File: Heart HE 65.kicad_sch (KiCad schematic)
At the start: 61 parts, among them J6 Conn_01x04, SW1 SW_Push, U1 PRTR5V0U2X, U19 AP2112K-3.3, U27 AT32F405KxU7-4, U63 AMS1117-3.3, U85 TPS63001, Y1 12Mhz (15p)

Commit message: Fix Component order part overwrite
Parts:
- C165, C20, C21, C25, C26, C32, C6, C8: LCSC C52923 -> (none)
- USB1: LCSC Part Number C165948 -> (none)
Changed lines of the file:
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@@
 			)
 		)
-		(property "LCSC" "C52923"
-			(at 140.97 139.7 0)
-			(effects
-				(font
-					(size 1.27 1.27)
-				)
-				(hide yes)
-			)
-		)
 		(pin "1"
 		)
@@
 			)
 		)
-		(property "LCSC" "C52923"
-			(at 151.13 139.7 0)
-			(effects
-				(font
-					(size 1.27 1.27)
-				)
-				(hide yes)
-			)
-		)
 		(pin "1"
 		)
@@
 			)
 		)
-		(property "LCSC" "C52923"
-			(at 217.17 105.41 0)
-			(effects
-				(font
-					(size 1.27 1.27)
-				)
-				(hide yes)
-			)
-		)
 		(pin "1"
 		)
@@
 			)
 		)
-		(property "LCSC" "C52923"
-			(at 260.985 99.695 0)
-			(effects
-				(font
-					(size 1.27 1.27)
-				)
-				(hide yes)
-			)
-		)
 		(pin "1"
 		)
@@
 			)
 		)
-		(property "LCSC" "C52923"
-			(at 153.67 153.67 0)
-			(effects
-				(font
-					(size 1.27 1.27)
-				)
-				(hide yes)
-			)
-		)
 		(pin "1"
 		)
@@
 			)
 		)
-		(property "LCSC" "C52923"
-			(at 158.75 153.67 0)
-			(effects
-				(font
-					(size 1.27 1.27)
-				)
-				(hide yes)
-			)
-		)
 		(pin "1"
 		)
@@
 			)
 		)
-		(property "LCSC" "C52923"
-			(at 137.16 186.69 0)
-			(effects
-				(font
-					(size 1.27 1.27)
-				)
-				(hide yes)
-			)
-		)
 		(pin "1"
 		)
@@
 			)
 		)
-		(property "LCSC" "C52923"
-			(at 162.56 186.69 0)
-			(effects
-				(font
-					(size 1.27 1.27)
-				)
-				(hide yes)
-			)
-		)
 		(pin "1"
 		)
@@
 			)
 		)
-		(property "LCSC" "C52923"
-			(at 257.175 99.695 0)
-			(effects
-				(font
-					(size 1.27 1.27)
-				)
-				(hide yes)
-			)
-		)
 		(pin "1"
 		)
@@
 			)
 		)
-		(property "LCSC" "C52923"
-			(at 200.025 150.495 0)
-			(effects
-				(font
-					(size 1.27 1.27)
-				)
-				(hide yes)
-			)
-		)
 		(pin "1"
 		)
@@
 			)
 		)
-		(property "LCSC" "C52923"
-			(at 181.61 150.495 0)
-			(effects
-				(font
-					(size 1.27 1.27)
-				)
-				(hide yes)
-			)
-		)
 		(pin "1"
 		)
@@
 			)
 		)
-		(property "LCSC Part Number" "C165948"
-			(at 22.86 199.39 0)
-			(effects
-				(font
-					(size 1.27 1.27)
-				)
-				(hide yes)
-			)
-		)
 		(pin "1"
 		)
@@
 			)
 		)
-		(property "LCSC" "C52923"
-			(at 210.82 96.52 0)
-			(effects
-				(font
-					(size 1.27 1.27)
-				)
-				(hide yes)
-			)
-		)
 		(pin "1"
 		)
@@
 			(at 146.05 139.7 0)
 			(effects
-				(font
-					(size 1.27 1.27)
-				)
-				(hide yes)
-			)
-		)
-		(property "LCSC" "C52923"
-			(at 146.05 139.7 0)
-			(effects

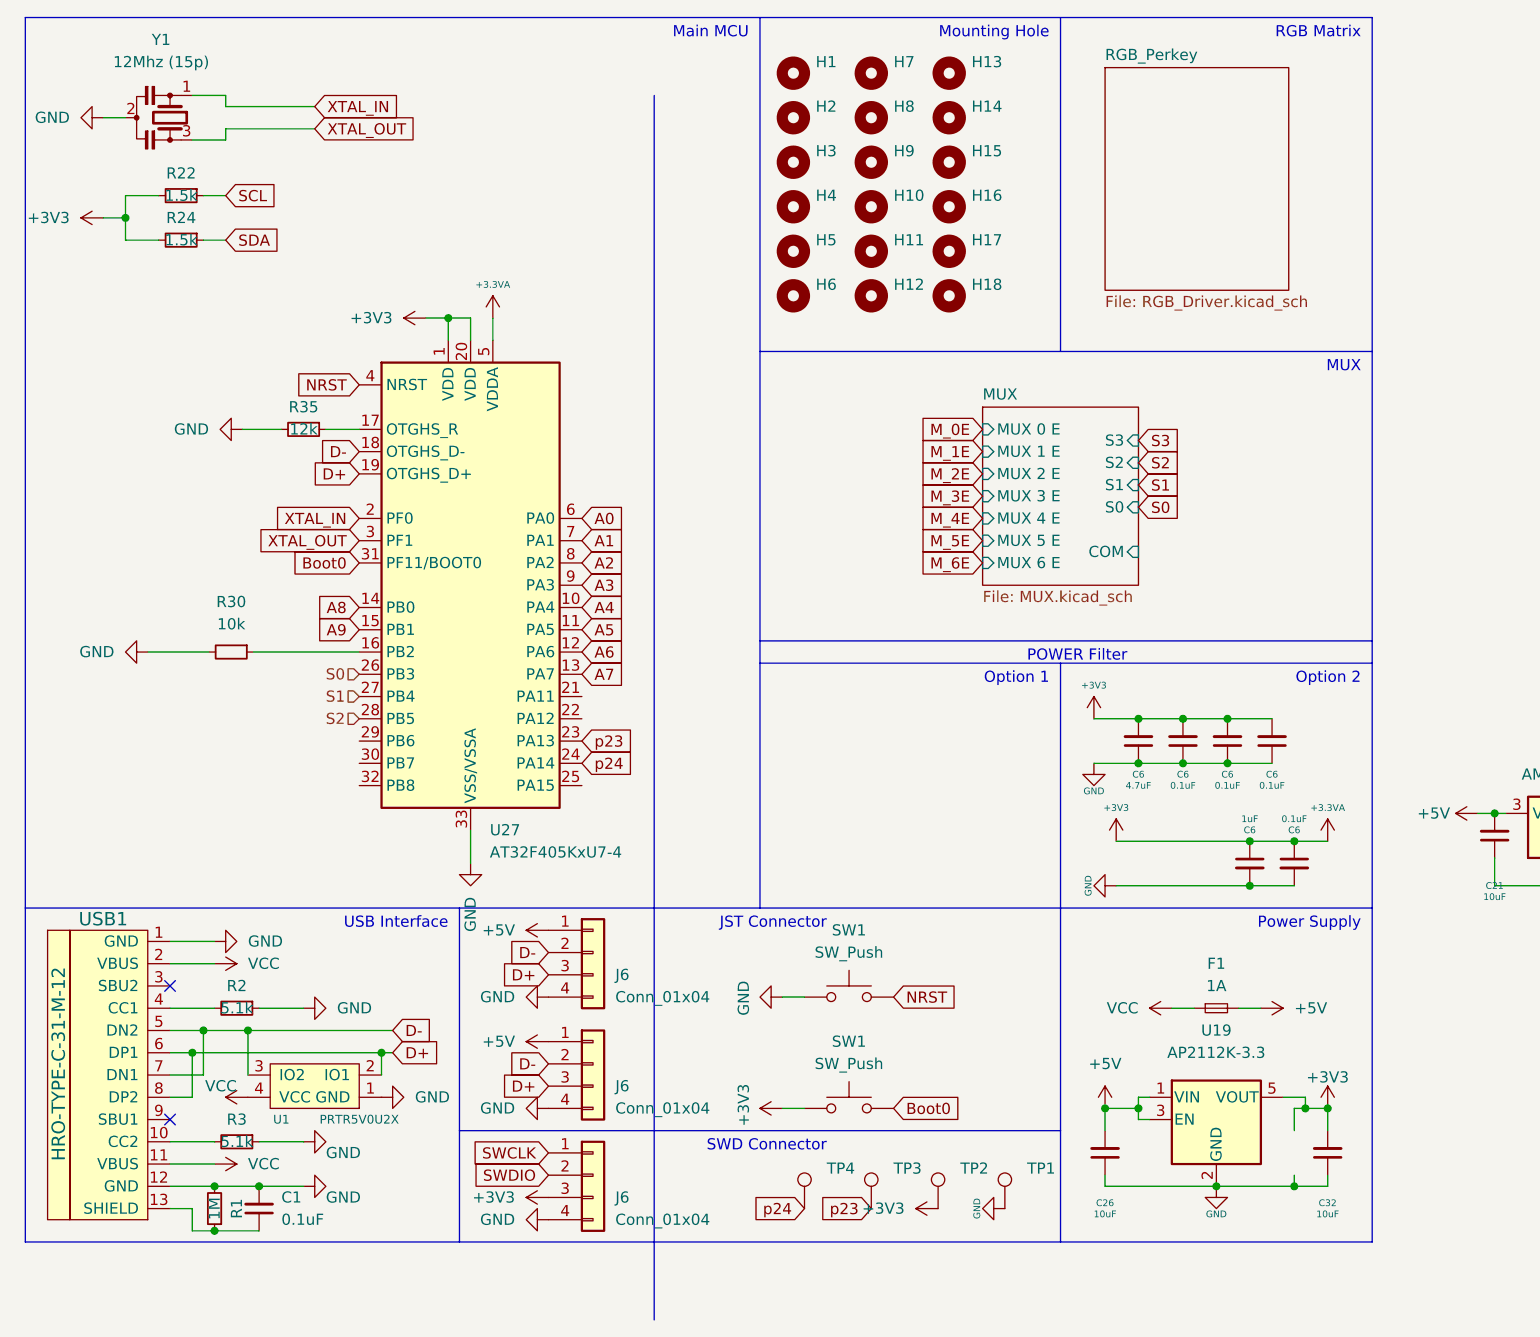
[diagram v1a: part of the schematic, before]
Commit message: a
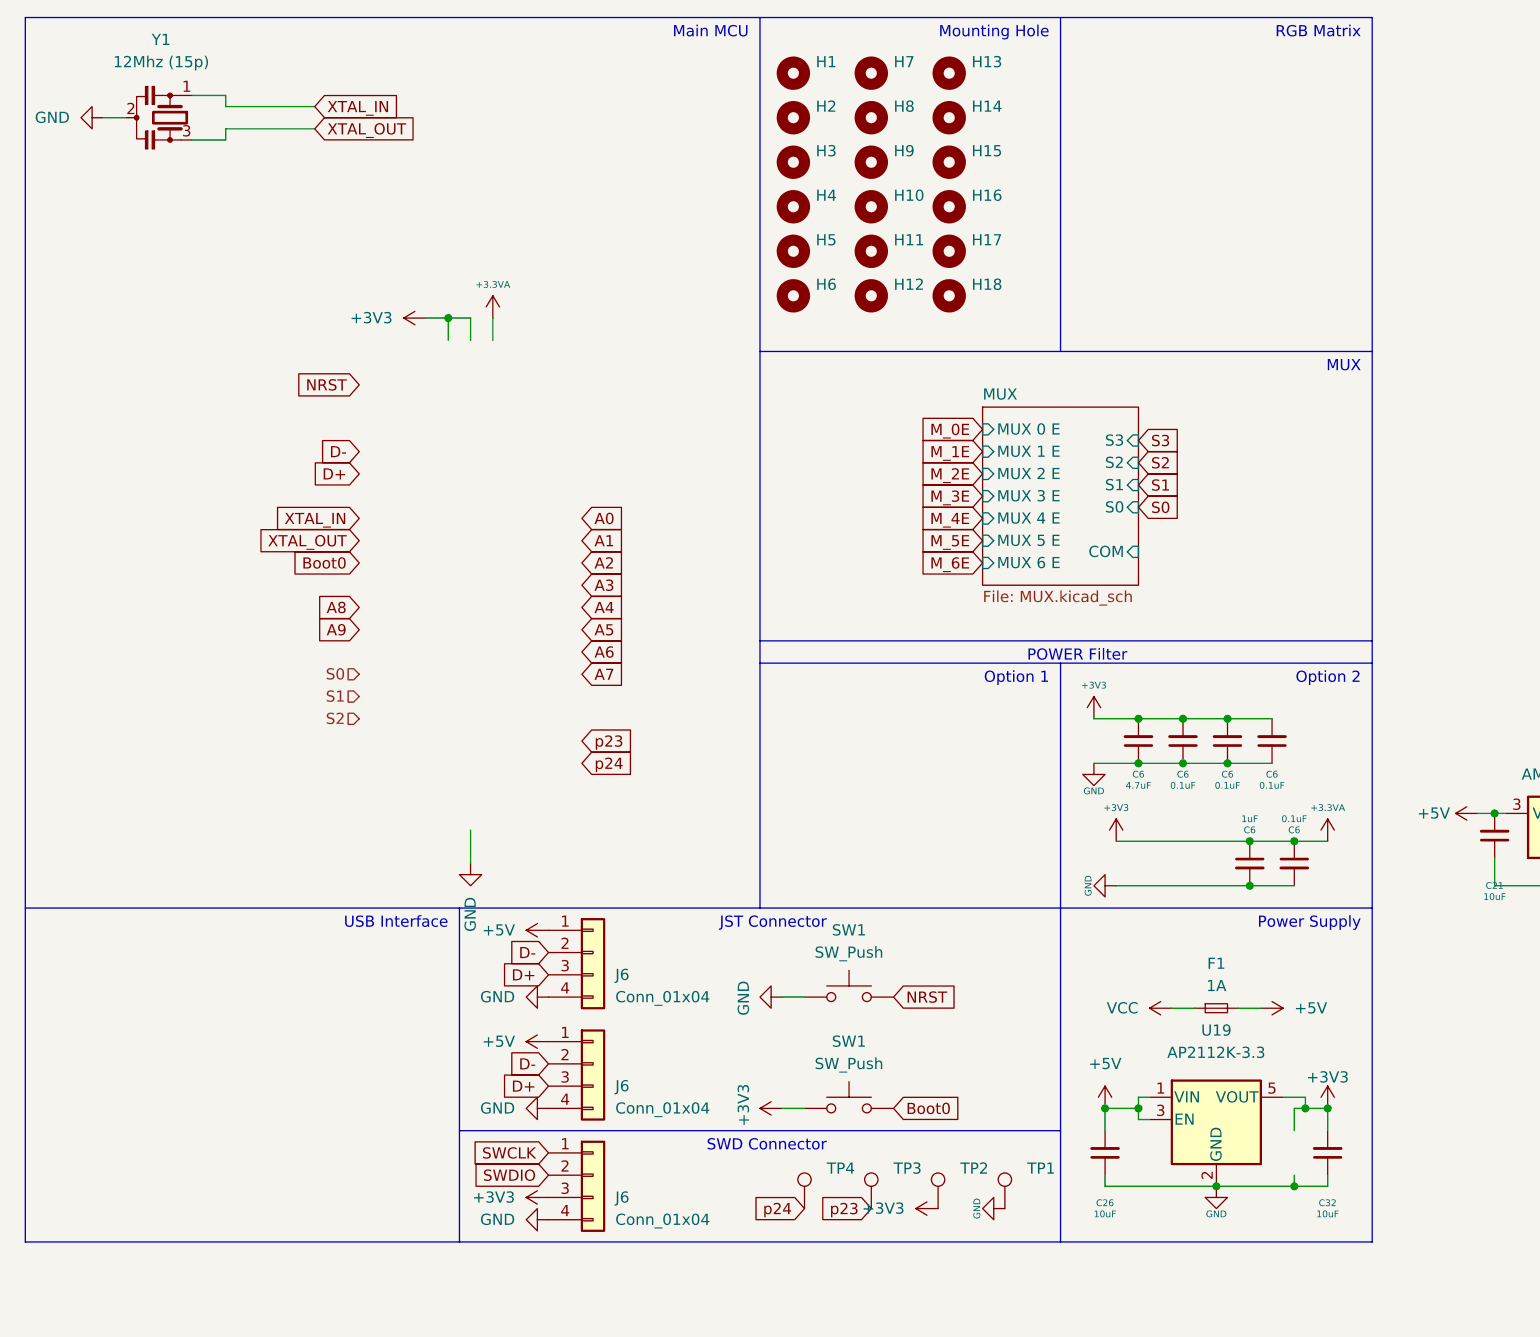
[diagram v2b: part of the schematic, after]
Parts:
- removed C1: 0.1uF, Common_Footprint:C_0402, symbol Device:C_Small
- removed R1: 1M, Common_Footprint:R_0402, symbol Device:R_Small
- removed R2, R3: 5.1k, Common_Footprint:R_0402, symbol Device:R_Small
- removed R22, R24: 1.5k, Common_Footprint:R_0402, symbol Device:R_Small
- removed R30: 10k, Common_Footprint:R_0402, symbol Device:R_Small
- removed R35: 12k, Common_Footprint:R_0402, symbol Device:R_Small
- removed U1: PRTR5V0U2X, symbol random-keyboard-parts:PRTR5V0U2X
- removed U27: AT32F405KxU7-4, Package_DFN_QFN:QFN-32-1EP_4x4mm_P0.4mm_EP2.9x2.9mm_ThermalVias, symbol MCU_Artery_AT32F40:AT32F405KxU7-4
- removed USB1: HRO-TYPE-C-31-M-12, Common_Footprint:HRO-TYPE-C-31-M-12-Assembly, symbol horrortroll_lib:HRO-TYPE-C-31-M-12
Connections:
- no-connect marks 2 -> 0
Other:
- removed sheet RGB_Perkey

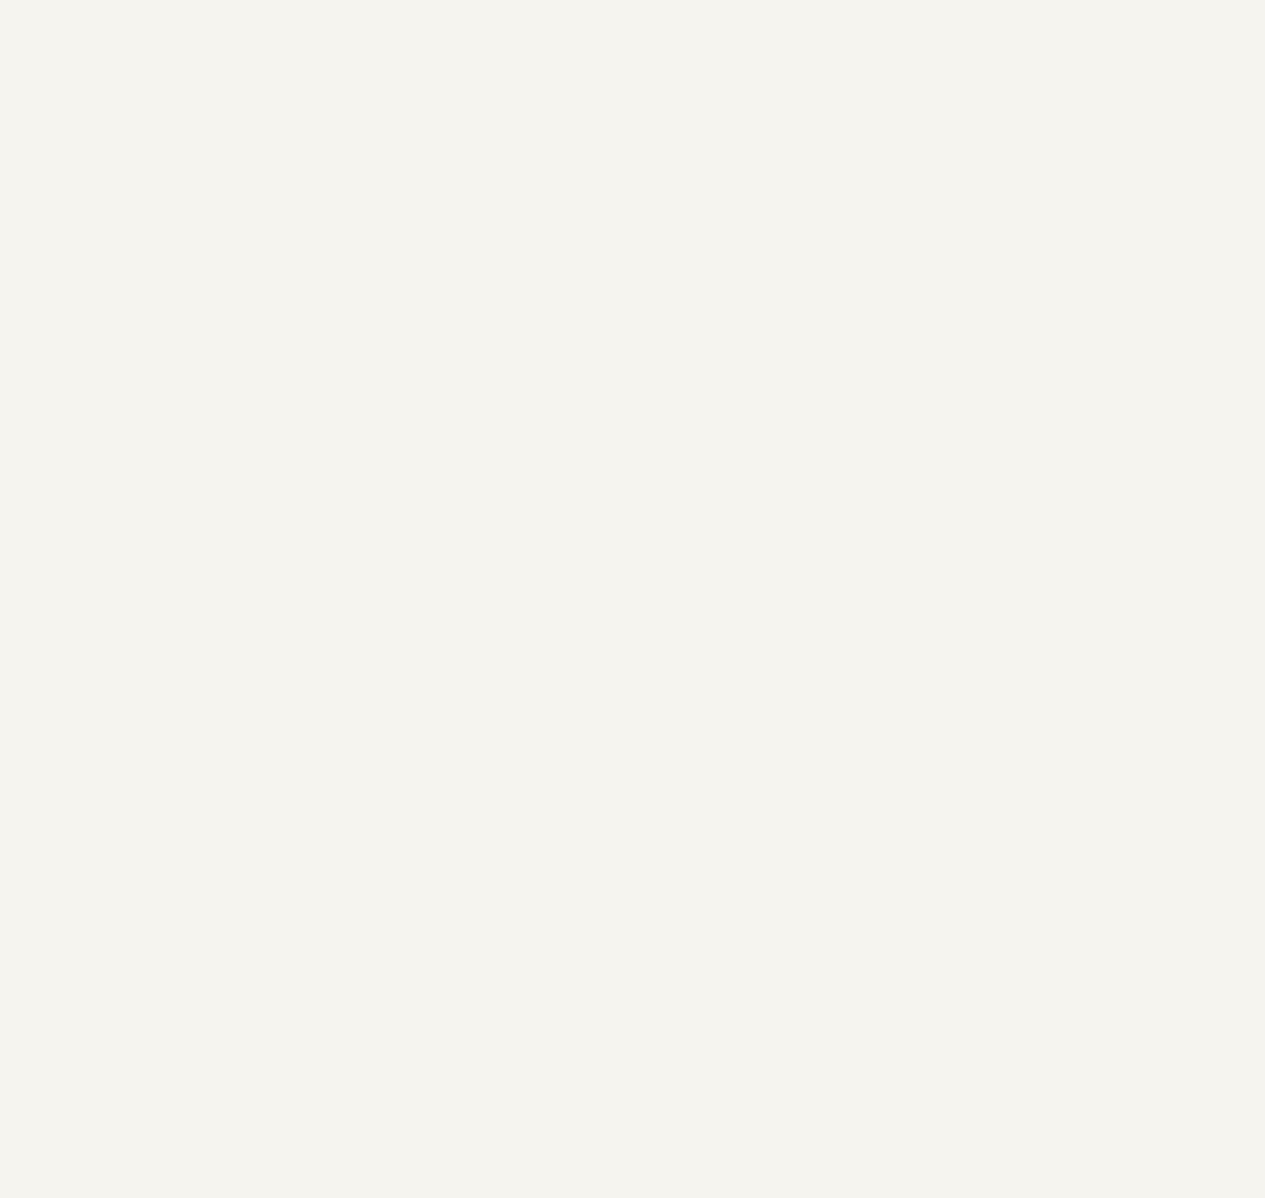
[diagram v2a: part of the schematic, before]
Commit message: a
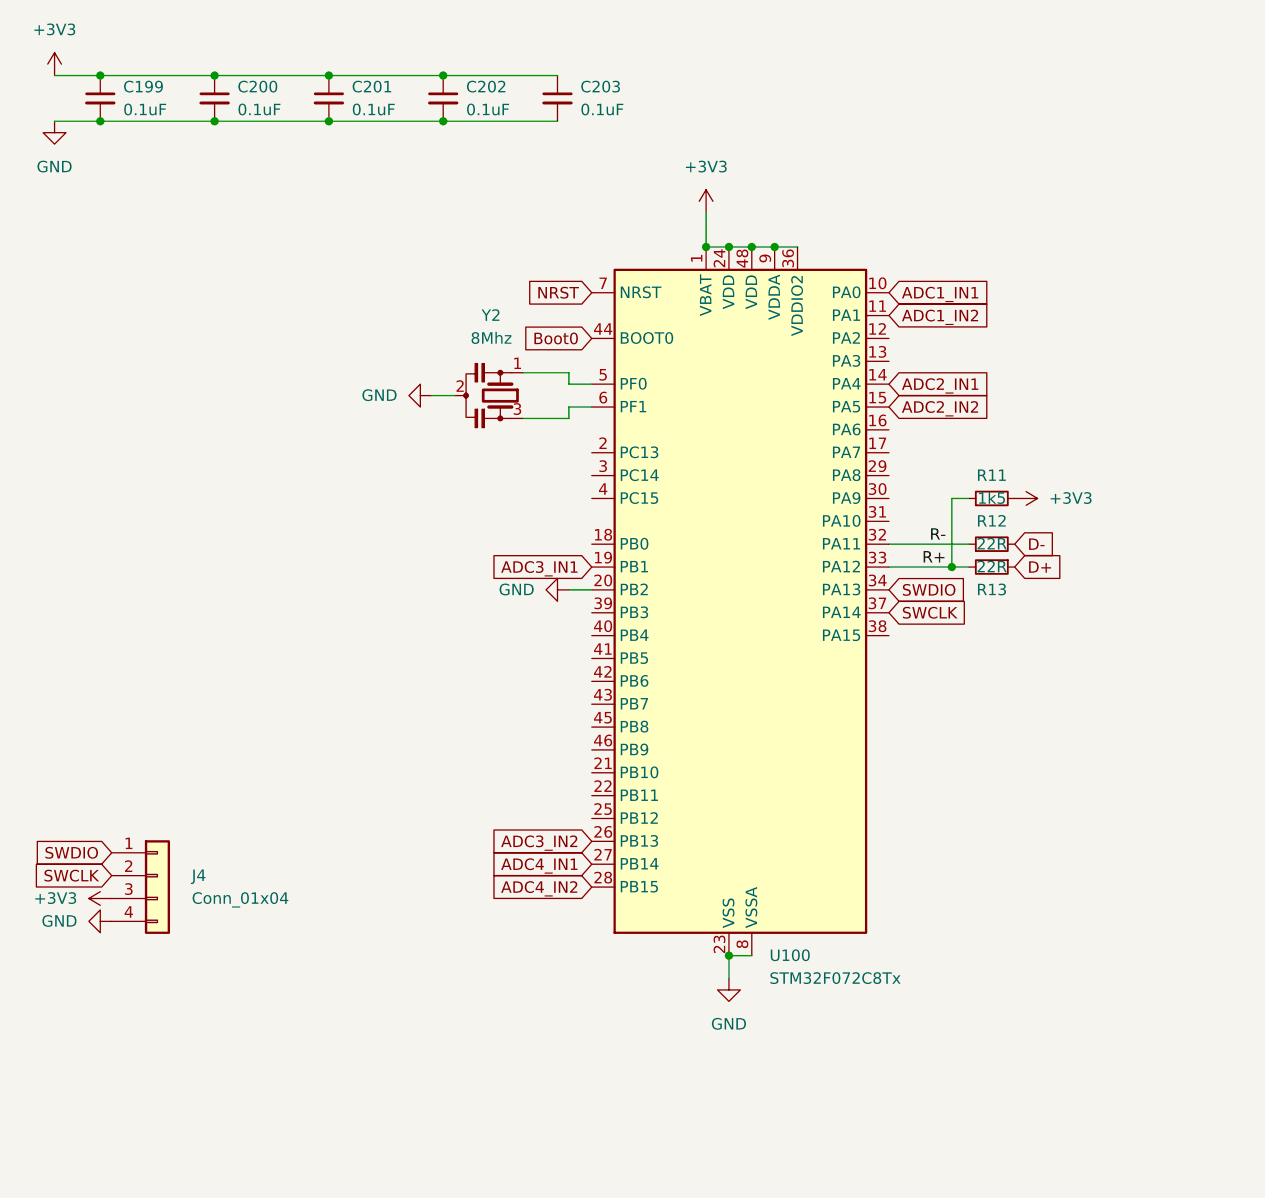
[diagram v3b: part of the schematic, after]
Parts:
- added C199, C200, C201, C202, C203: 0.1uF, Common_Footprint:C_0402, symbol Device:C_Small
- added J4: Conn_01x04, Connector_PinHeader_2.54mm:PinHeader_1x04_P2.54mm_Vertical, symbol Connector_Generic:Conn_01x04
- added R11: 1k5, Common_Footprint:R_0402, symbol Device:R_Small
- added R12, R13: 22R, Common_Footprint:R_0402, symbol Device:R_Small
- added U100: STM32F072C8Tx, Package_QFP:LQFP-48_7x7mm_P0.5mm, symbol MCU_ST_STM32F0:STM32F072C8Tx
- added Y2: 8Mhz, Crystal:Resonator_SMD_Murata_CSTxExxV-3Pin_3.0x1.1mm, symbol Device:Resonator_Small
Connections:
- net +3.3VA: now also C199.1, C200.1, C201.1, C202.1, C203.1, J4.3 (Pin_3), R11.2, U100.1 (VBAT), U100.24 (VDD), U100.36 (VDDIO2), U100.48 (VDD), U100.9 (VDDA)
- net Boot0: now also U100.44 (BOOT0)
- net D+: now also R13.1
- net D-: now also R12.2
- net GND: now also C199.2, C200.2, C201.2, C202.2, C203.2, J4.4 (Pin_4), U100.20 (PB2), U100.23 (VSS), U100.35 (VSS), U100.47 (VSS), U100.8 (VSSA), Y2.2
- net NRST: now also U100.7 (NRST)
- net SWCLK: now also J4.2 (Pin_2), U100.37 (PA14)
- net SWDIO: now also J4.1 (Pin_1), U100.34 (PA13)
- new net: U100.5 (PF0), Y2.1
- new net: U100.6 (PF1), Y2.3
- new net ADC1_IN1: U100.10 (PA0)
- new net ADC1_IN2: U100.11 (PA1)
- new net ADC2_IN1: U100.14 (PA4)
- new net ADC2_IN2: U100.15 (PA5)
- new net ADC3_IN1: U100.19 (PB1)
- new net ADC3_IN2: U100.26 (PB13)
- new net ADC4_IN1: U100.27 (PB14)
- new net ADC4_IN2: U100.28 (PB15)
- new net R+: R11.1, R13.2, U100.33 (PA12)
- new net R-: R12.1, U100.32 (PA11)
